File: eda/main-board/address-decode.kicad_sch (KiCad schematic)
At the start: 29 parts, among them J6 CS_leds, U10 74HCT00, U12 74HCT32, U5 74HCT138, U6 74HCT32, U7 74HCT08, U8 74HCT30, U9 74HCT139

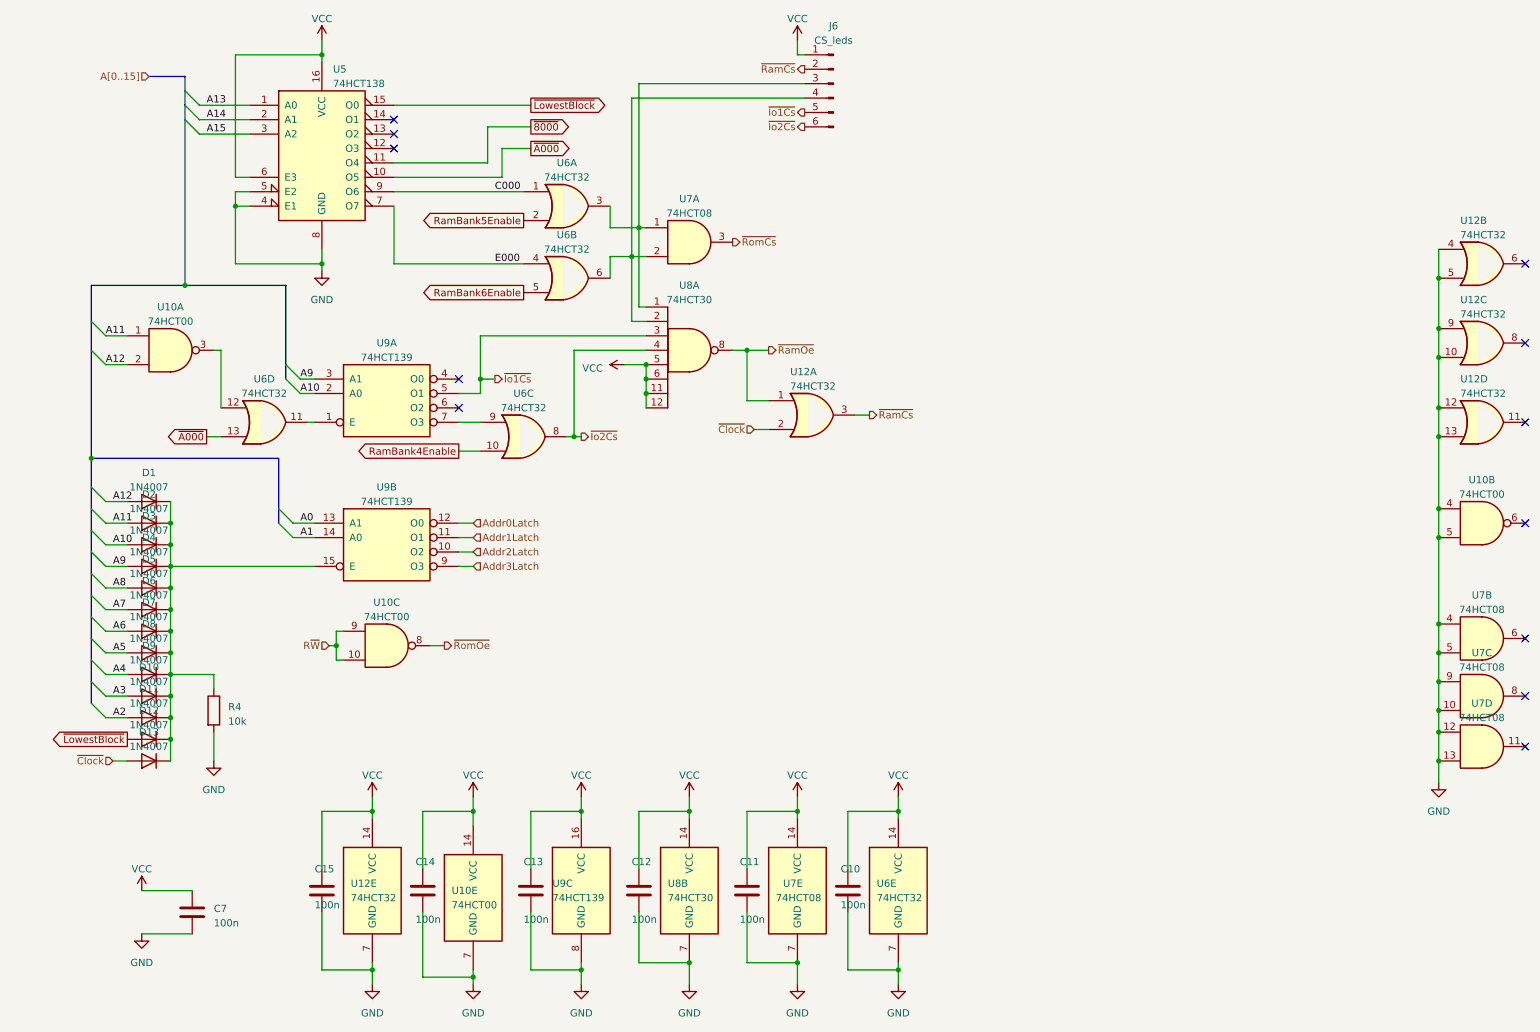
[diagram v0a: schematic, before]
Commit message: Did stuff
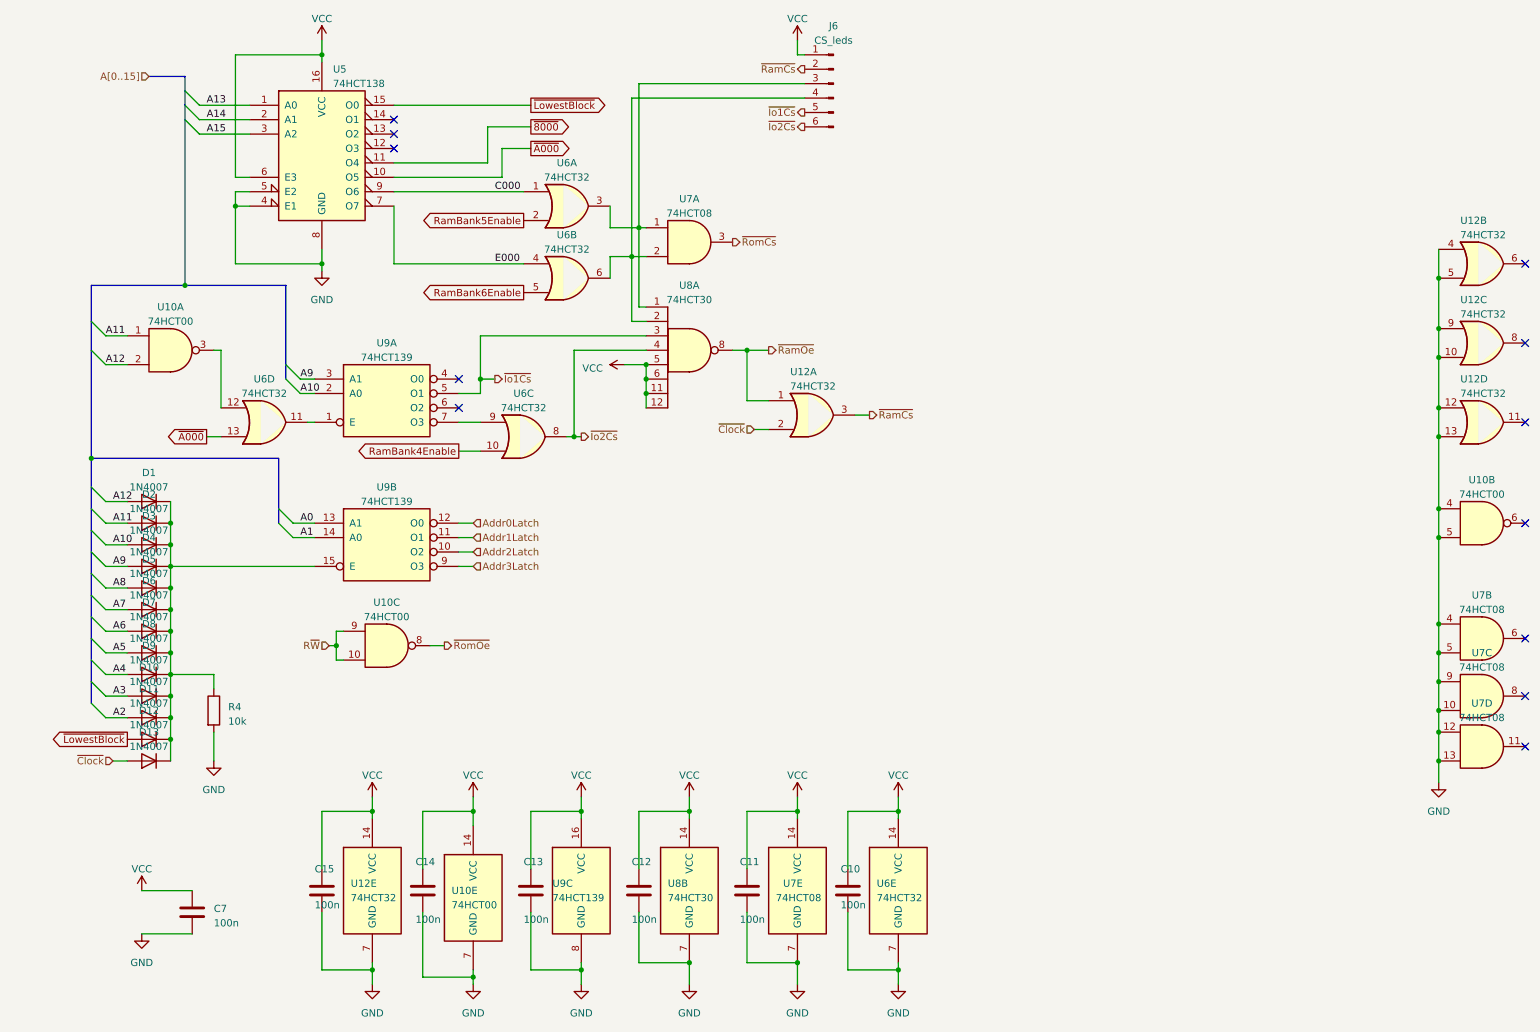
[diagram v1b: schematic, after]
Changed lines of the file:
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@@
 (kicad_sch
-	(version 20231120)
+	(version 20250114)
 	(generator "eeschema")
-	(generator_version "8.0")
+	(generator_version "9.0")
 	(paper "A4")
 	(junction
@@
 	(label "A11"
 		(at 24.13 110.49 0)
-		(fields_autoplaced yes)
 		(effects
 			(font
@@
 	(label "A12"
 		(at 22.86 82.55 0)
-		(fields_autoplaced yes)
 		(effects
 			(font
@@
 	(label "C000"
 		(at 91.44 52.07 0)
-		(fields_autoplaced yes)
 		(effects
 			(font
@@
 	(label "A2"
 		(at 24.13 144.78 0)
-		(fields_autoplaced yes)
 		(effects
 			(font
@@
 	(label "A3"
 		(at 24.13 140.97 0)
-		(fields_autoplaced yes)
 		(effects
 			(font
@@
 	(label "A8"
 		(at 24.13 121.92 0)
-		(fields_autoplaced yes)
 		(effects
 			(font
@@
 	(label "A0"
 		(at 57.15 110.49 0)
-		(fields_autoplaced yes)
 		(effects
 			(font
@@
 	(label "A11"
 		(at 22.86 77.47 0)
-		(fields_autoplaced yes)
 		(effects
 			(font
@@
 	(label "A7"
 		(at 24.13 125.73 0)
-		(fields_autoplaced yes)
 		(effects
 			(font
@@
 	(label "A5"
 		(at 24.13 133.35 0)
-		(fields_autoplaced yes)
 		(effects
 			(font
@@
 	(label "A12"
 		(at 24.13 106.68 0)
-		(fields_autoplaced yes)
 		(effects
 			(font
@@
 	(label "A10"
 		(at 57.15 87.63 0)
-		(fields_autoplaced yes)
 		(effects
 			(font
@@
 	(label "A9"
 		(at 57.15 85.09 0)
-		(fields_autoplaced yes)
 		(effects
 			(font
@@
 	(label "A6"
 		(at 24.13 129.54 0)
-		(fields_autoplaced yes)
 		(effects
 			(font
@@
 	(label "A13"
 		(at 40.64 36.83 0)
-		(fields_autoplaced yes)
 		(effects
 			(font
@@
 	(label "A9"
 		(at 24.13 118.11 0)
-		(fields_autoplaced yes)
 		(effects
 			(font
@@
 	(label "A4"
 		(at 24.13 137.16 0)
-		(fields_autoplaced yes)
 		(effects
 			(font
@@
 	(label "A15"
 		(at 40.64 41.91 0)
-		(fields_autoplaced yes)
 		(effects
 			(font
@@
 	(label "E000"
 		(at 91.44 64.77 0)
-		(fields_autoplaced yes)
 		(effects
 			(font
@@
 	(label "A14"
 		(at 40.64 39.37 0)
-		(fields_autoplaced yes)
 		(effects
 			(font
@@
 	(label "A1"
 		(at 57.15 113.03 0)
-		(fields_autoplaced yes)
 		(effects
 			(font
@@
 	(label "A10"
 		(at 24.13 114.3 0)
-		(fields_autoplaced yes)
 		(effects
 			(font
@@
 		(shape output)
 		(at 146.05 30.48 180)
-		(fields_autoplaced yes)
 		(effects
 			(font
@@
 		(shape input)
 		(at 62.23 132.08 180)
-		(fields_autoplaced yes)
 		(effects
 			(font
@@
 		(shape output)
 		(at 133.35 60.96 0)
-		(fields_autoplaced yes)
 		(effects
 			(font
@@
 		(shape input)
 		(at 87.63 113.03 0)
-		(fields_autoplaced yes)
 		(effects
 			(font
@@
 		(shape output)
 		(at 106.68 95.25 0)
-		(fields_autoplaced yes)
 		(effects
 			(font
@@
 		(shape input)
 		(at 87.63 110.49 0)
-		(fields_autoplaced yes)
 		(effects
 			(font
@@
 		(shape output)
 		(at 157.48 91.44 0)
-		(fields_autoplaced yes)
 		(effects
 			(font
@@
 		(shape input)
 		(at 87.63 115.57 0)
-		(fields_autoplaced yes)
 		(effects
 			(font
@@
 		(shape input)
 		(at 24.13 152.4 180)
-		(fields_autoplaced yes)
 		(effects
 			(font
@@
 		(shape input)
 		(at 87.63 118.11 0)
-		(fields_autoplaced yes)
 		(effects
 			(font
@@
 		(shape output)
 		(at 139.7 80.01 0)
-		(fields_autoplaced yes)
 		(effects
 			(font
@@
 		(shape input)
 		(at 30.48 31.75 180)
-		(fields_autoplaced yes)
 		(effects
 			(font
@@
 		(shape output)
 		(at 82.55 132.08 0)
-		(fields_autoplaced yes)
 		(effects
 			(font
@@
 		(shape output)
 		(at 91.44 85.09 0)
-		(fields_autoplaced yes)
 		(effects
 			(font
@@
 		(shape output)
 		(at 146.05 38.1 180)
-		(fields_autoplaced yes)
 		(effects
 			(font
@@
 		(shape input)
 		(at 137.16 93.98 180)
-		(fields_autoplaced yes)
 		(effects
 			(font
@@
 		(shape output)
 		(at 146.05 40.64 180)
-		(fields_autoplaced yes)
-		(effects
-			(font
+		(effects
+			(font
